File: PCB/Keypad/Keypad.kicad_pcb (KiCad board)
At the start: 2 copper layers, 70 x 70 mm, 26 parts, among them J1 Keypad, J4 TC2030-USB-NL-DS, U1 SP3485, U3 ESP32-S3-MINI-1, U4 QR, U5 MD8942

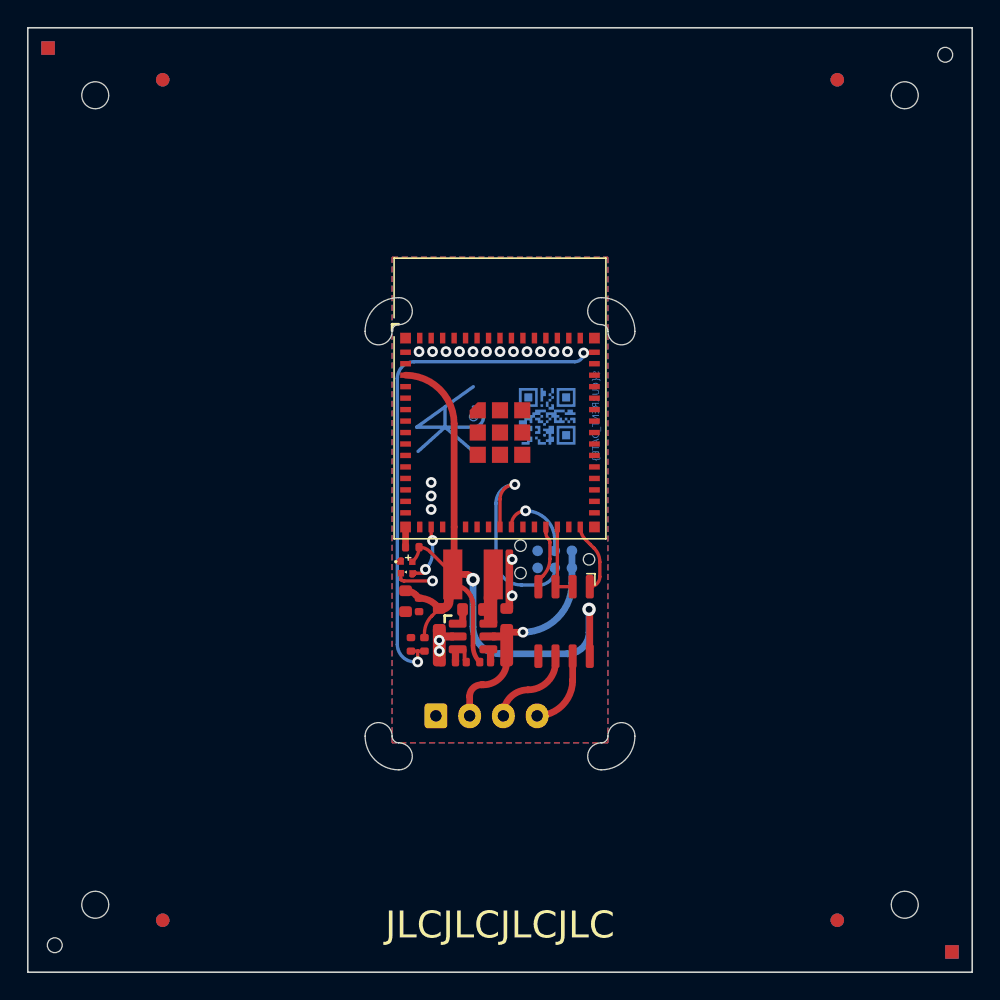
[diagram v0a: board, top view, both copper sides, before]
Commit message: Cannot make production files, FFS
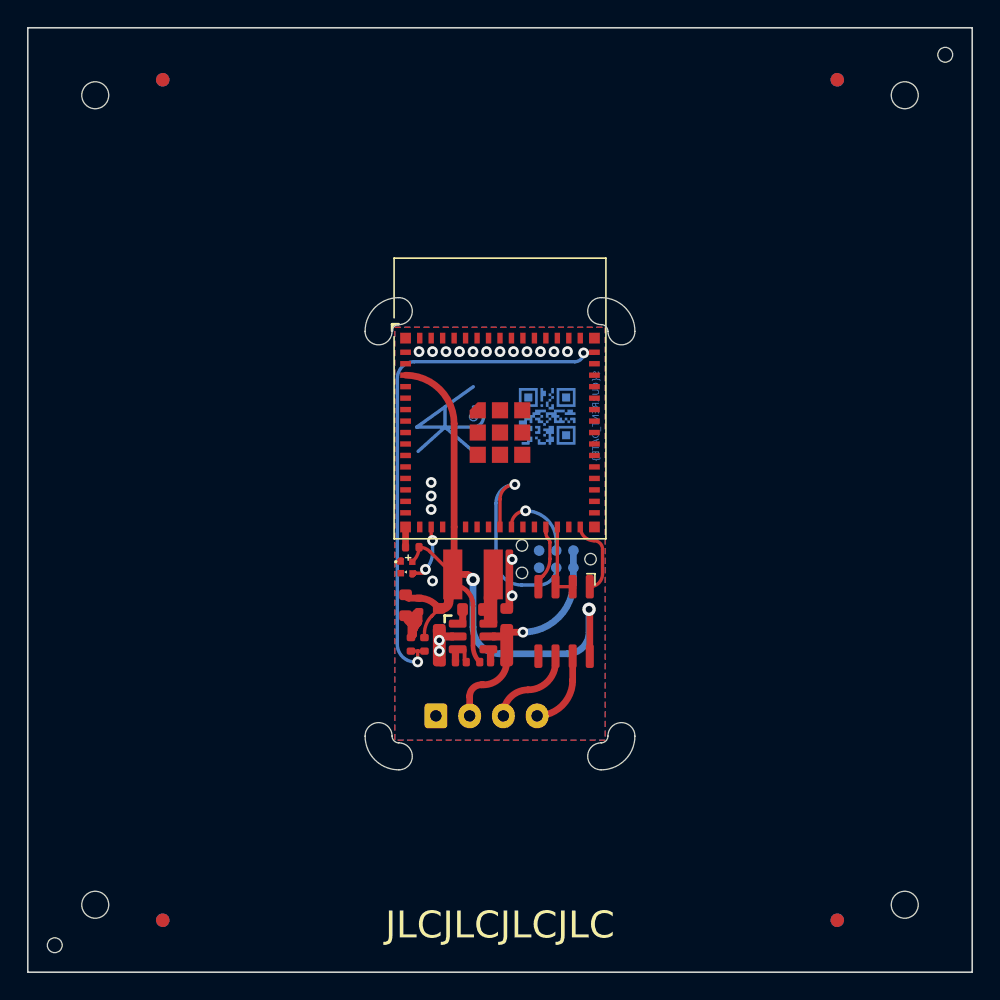
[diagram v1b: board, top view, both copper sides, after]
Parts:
- moved C3 0.30 mm to (93.0, 107.8)
- moved J4 0.11 mm to (104.2, 104.4)
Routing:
- net GND: track 4.35 -> 8.94 mm
- net RX: track 5.29 -> 5.80 mm
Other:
- board text added: "R E"
- board text added: "R H"
- board text added: "R L"
